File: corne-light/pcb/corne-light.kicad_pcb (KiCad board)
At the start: 2 copper layers, 275.5 x 105.6 mm, 43 parts, among them SW22 SW_PUSH, SW23 SW_PUSH, SW24 SW_PUSH, SW25 SW_PUSH, SW26 SW_PUSH, SW27 SW_PUSH, SW28 SW_PUSH, SW29 SW_PUSH, SW30 SW_PUSH, SW31 SW_PUSH, SW32 SW_PUSH, SW33 SW_PUSH, SW34 SW_PUSH, SW35 SW_PUSH, SW36 SW_PUSH, SW37 SW_PUSH, SW38 SW_PUSH, SW39 SW_PUSH, SW40 SW_PUSH, SW41 SW_PUSH, SW42 SW_PUSH, U1 nice_nano

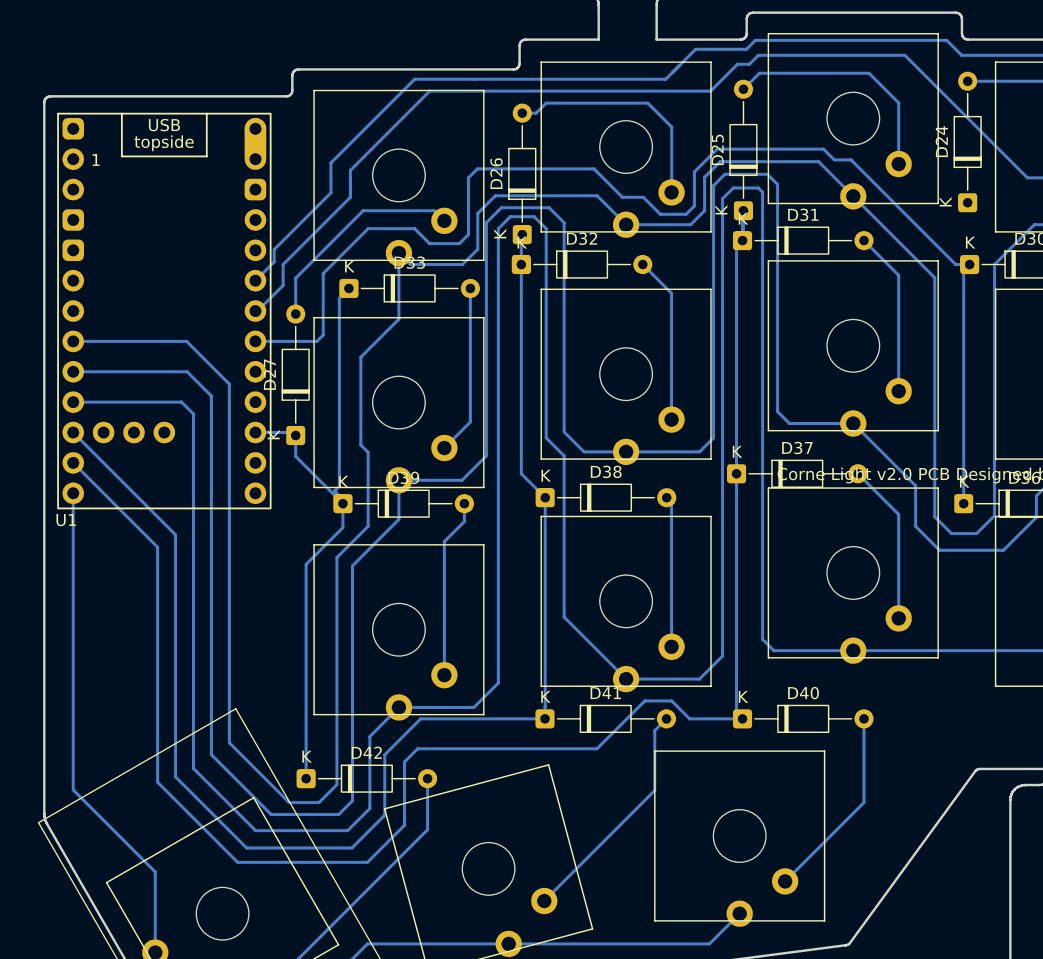
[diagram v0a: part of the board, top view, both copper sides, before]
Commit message: Improve tracks
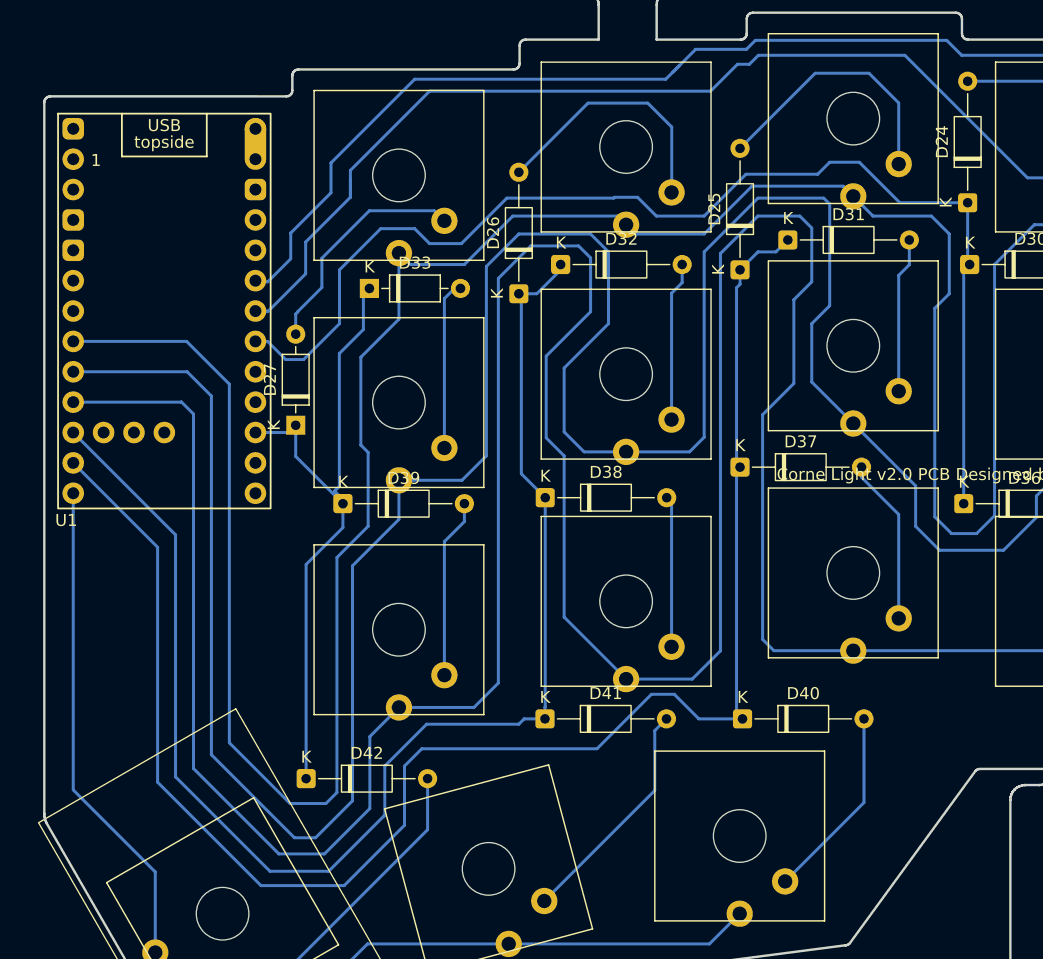
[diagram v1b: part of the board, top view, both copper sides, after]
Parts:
- D27, D33: footprint Diode_THT:D_DO-35_SOD27_P10.16mm_Horizontal -> Diode_THT:D_DO-35_SOD27_P7.62mm_Horizontal
- moved D25 4.95 mm to (212.2, 51.4)
- moved D26 4.95 mm to (193.7, 53.4)
- moved D31 3.79 mm to (216.2, 48.9)
- moved D32 3.29 mm to (197.2, 51.0)
- moved D33 1.71 mm to (181.2, 53.0)
- moved D27 0.86 mm to (175.1, 64.4)
- moved D37 0.63 mm to (212.2, 67.9)
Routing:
- net row1_r: track 292.8 -> 289.1 mm
- net col2_r: track 102.2 -> 98.9 mm
- net Net-(D26-A): track 19.2 -> 21.5 mm
- net Net-(D25-A): track 19.7 -> 22.0 mm
- net col5_r: track 53.9 -> 55.8 mm
- net row0_r: track 347.4 -> 345.8 mm
- net Net-(D27-A): track 18.1 -> 19.5 mm
- net Net-(D31-A): track 13.8 -> 13.0 mm
- net col0_r: track 149.2 -> 149.9 mm
- net Net-(D32-A): track 14.0 -> 13.3 mm
- net col1_r: track 124.1 -> 124.7 mm
